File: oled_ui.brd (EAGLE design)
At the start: 77.5 x 19.4 mm, 30 parts

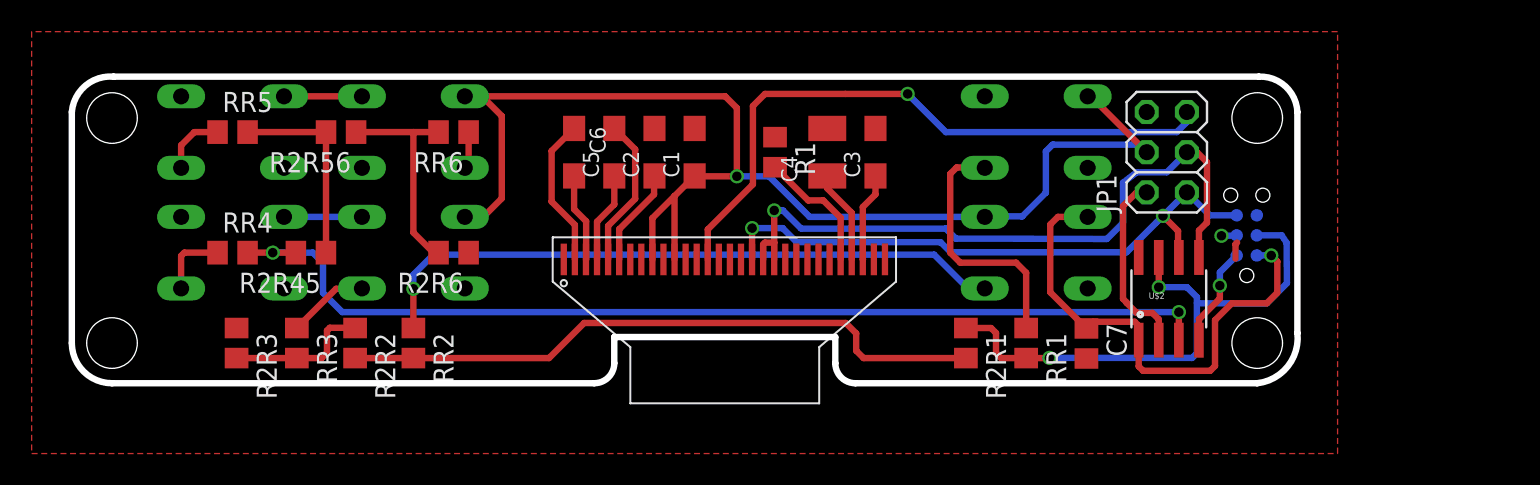
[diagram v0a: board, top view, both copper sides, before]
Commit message: updates
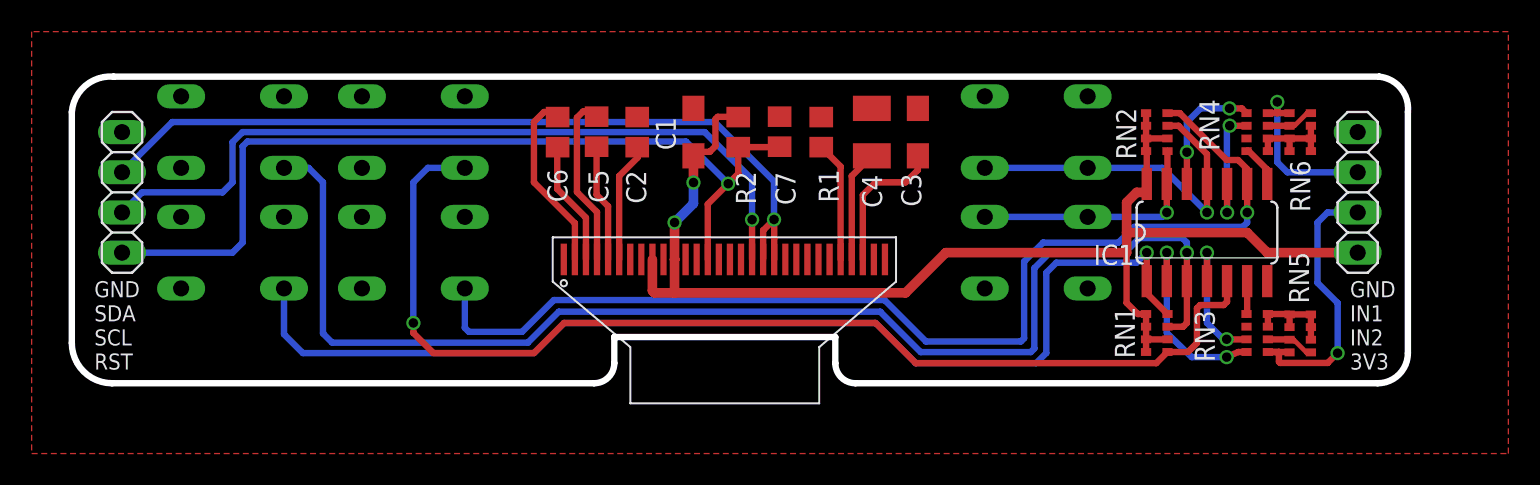
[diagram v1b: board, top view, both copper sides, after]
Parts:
- removed J1: (no value), tag-connect:TC2030-MCP-NL
- removed R2R1, R2R2, R2R3, R2R45, R2R56, R2R6, RR1, RR2, RR3, RR4, RR5, RR6: (no value), rcl:R0805
- removed U$2: PIC12F1822SO08, jasons_stuff:SO08
- added IC1: 74HC14D, 74xx-eu:SO14
- added JP2: (no value), pinhead:1X04
- added R2: (no value), rcl:R0805
- added RN1, RN2, RN3, RN4, RN5, RN6: (no value), resistor-dil:CAY16
- C2, C5, C6: device resistor:SMC_A -> rcl:C0805
- JP1: device pinhead:2X03 -> pinhead:1X04
- moved JP1 66.1 mm to (3.17, 14.0)
- moved C7 23.6 mm to (44.7, 17.8)
- moved S5 13.7 mm to (21.6, 10.2)
- moved S6 13.7 mm to (10.2, 10.2)
- moved S3 7.62 mm to (21.6, 17.8)
- moved S4 7.62 mm to (10.2, 17.8)
- moved R1 3.19 mm to (47.4, 17.8)
- moved C4 3.09 mm to (50.6, 17.8)
- moved C3 2.97 mm to (53.5, 17.8)
- moved C5 1.71 mm to (33.2, 17.8), turned to 270 degrees
- moved C2 1.68 mm to (35.7, 17.8)
- moved C6 1.64 mm to (30.7, 17.8)
- moved C1 1.27 mm to (39.3, 17.8)
- turned S2 to 0 degrees
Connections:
- removed net IRQ: JP1.2, U$2.2
- removed net OLED_RST: JP1.5, U$1.14
- removed net VDD: C1.+, C7.1, J1.2, JP1.4, S1.3, S1.4, S2.3, S2.4, S3.3, S3.4, S4.3, S4.4, S5.3, S5.4, S6.3, S6.4, U$1.11, U$1.9, U$2.1
- new net 3V3: C1.+, IC1.14, JP2.1, R2.2, RN1.2, RN1.5, RN1.6, RN1.7, RN1.8, RN2.2, RN2.5, RN2.6, RN2.7, RN2.8, U$1.11, U$1.9
- new net BUTTONS_OUT1: JP2.3, RN4.8, RN6.5
- new net BUTTONS_OUT2: JP2.2, RN3.5, RN5.8
- new net N$22: RN4.5, RN4.6, RN6.1, RN6.2, RN6.3, RN6.7, RN6.8
- new net N$23: RN3.6, RN5.1, RN5.7
- new net N$26: RN3.7, RN3.8, RN5.2, RN5.3, RN5.4, RN5.5, RN5.6
- new net RST: C7.2, JP1.1, R2.1, U$1.14
- net GND: now also C2.2, C7.1, IC1.7, JP1.4, JP2.4, RN3.2, RN4.3, S1.3, S1.4, S2.3, S2.4, S3.3, S3.4, S4.3, S4.4, S5.3, S5.4, S6.3, S6.4; no longer C2.-, C7.2, J1.3, JP1.6, R2R3.1, R2R6.1, U$2.8
- net N$1: now also C6.2; no longer C6.-
- net N$11: now also IC1.1, RN1.4, S6.2; no longer RR1.1, S1.1, S1.2
- net N$12: now also IC1.9, RN2.4, S5.2; no longer R2R45.2, RR4.2, U$2.3
- net N$13: now also IC1.11, RN2.3, S1.1, S1.2; no longer RR2.1, S2.1, S2.2
- net N$14: now also IC1.13, RN2.1, S2.1, S2.2; no longer RR6.1, S6.1, S6.2
- net N$15: now also IC1.12, RN4.1; no longer RR5.1, S5.1, S5.2
- net N$16: now also IC1.10, RN4.2; no longer RR4.1, S4.1, S4.2
- net N$17: now also IC1.8, RN4.4; no longer RR3.1, S3.1, S3.2
- net N$18: now also IC1.4, RN3.3; no longer J1.4, R2R1.1, RR1.2, U$2.7
- net N$19: now also IC1.2, RN3.4; no longer R2R1.2, R2R2.2, RR2.2
- net N$2: now also C6.1; no longer C6.+
- net N$20: now also IC1.6, RN3.1; no longer R2R2.1, R2R3.2, RR3.2
- net N$21: now also RN4.7, RN6.4, RN6.6; no longer J1.1, U$2.4
- net N$3: now also C5.1; no longer C5.+
- net N$4: now also C5.2; no longer C5.-
- net N$5: now also IC1.5, RN1.1, S3.2; no longer R2R56.1, R2R6.2, RR6.2
- net N$7: now also C2.1; no longer C2.+
- net N$9: now also IC1.3, RN1.3, S4.2; no longer R2R45.1, R2R56.2, RR5.2
- net SCL: now also JP1.2; no longer J1.5, JP1.1, U$2.6
- net SDA: no longer U$2.5
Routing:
- net VDD: track 123.7 -> 0.00 mm, vias 2 -> 0
- net 3V3: track 0.00 -> 81.9 mm, vias 0 -> 2
- net N$9: track 12.6 -> 81.6 mm, vias 0 -> 1
- net N$5: track 13.7 -> 71.1 mm, vias 0 -> 1
- net RST: track 0.00 -> 56.4 mm, vias 0 -> 1
- net N$11: track 16.2 -> 70.1 mm, vias 0 -> 1
- net OLED_RST: track 40.5 -> 0.00 mm, vias 1 -> 0
- net N$19: track 41.1 -> 12.6 mm, vias 0 -> 2
- net N$18: track 35.3 -> 9.32 mm
- net N$13: track 40.9 -> 22.1 mm
- net BUTTONS_OUT2: track 0.00 -> 18.3 mm, vias 0 -> 1
- net N$14: track 2.36 -> 15.5 mm, vias 0 -> 1
- net IRQ: track 11.9 -> 0.00 mm
- net BUTTONS_OUT1: track 0.00 -> 11.2 mm, vias 0 -> 1
- net SCL: track 38.6 -> 49.7 mm, vias 2 -> 1
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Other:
- board size 77.5 x 19.4 mm -> 84.5 x 19.4 mm
- board text added: "GND IN1 IN2 3V3"
- board text added: "GND SDA SCL RST"
- board text added: "TINY UI"
- board text added: "hotchk155"
- board text added: "rev2"
- board text added: "six4pix.com"
